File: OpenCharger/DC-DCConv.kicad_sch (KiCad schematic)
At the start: 10 parts, among them Q5 IPT015N10N5, Q6 IPT015N10N5, Q7 IPT015N10N5, Q9 IPT015N10N5, U4 IRS25606S

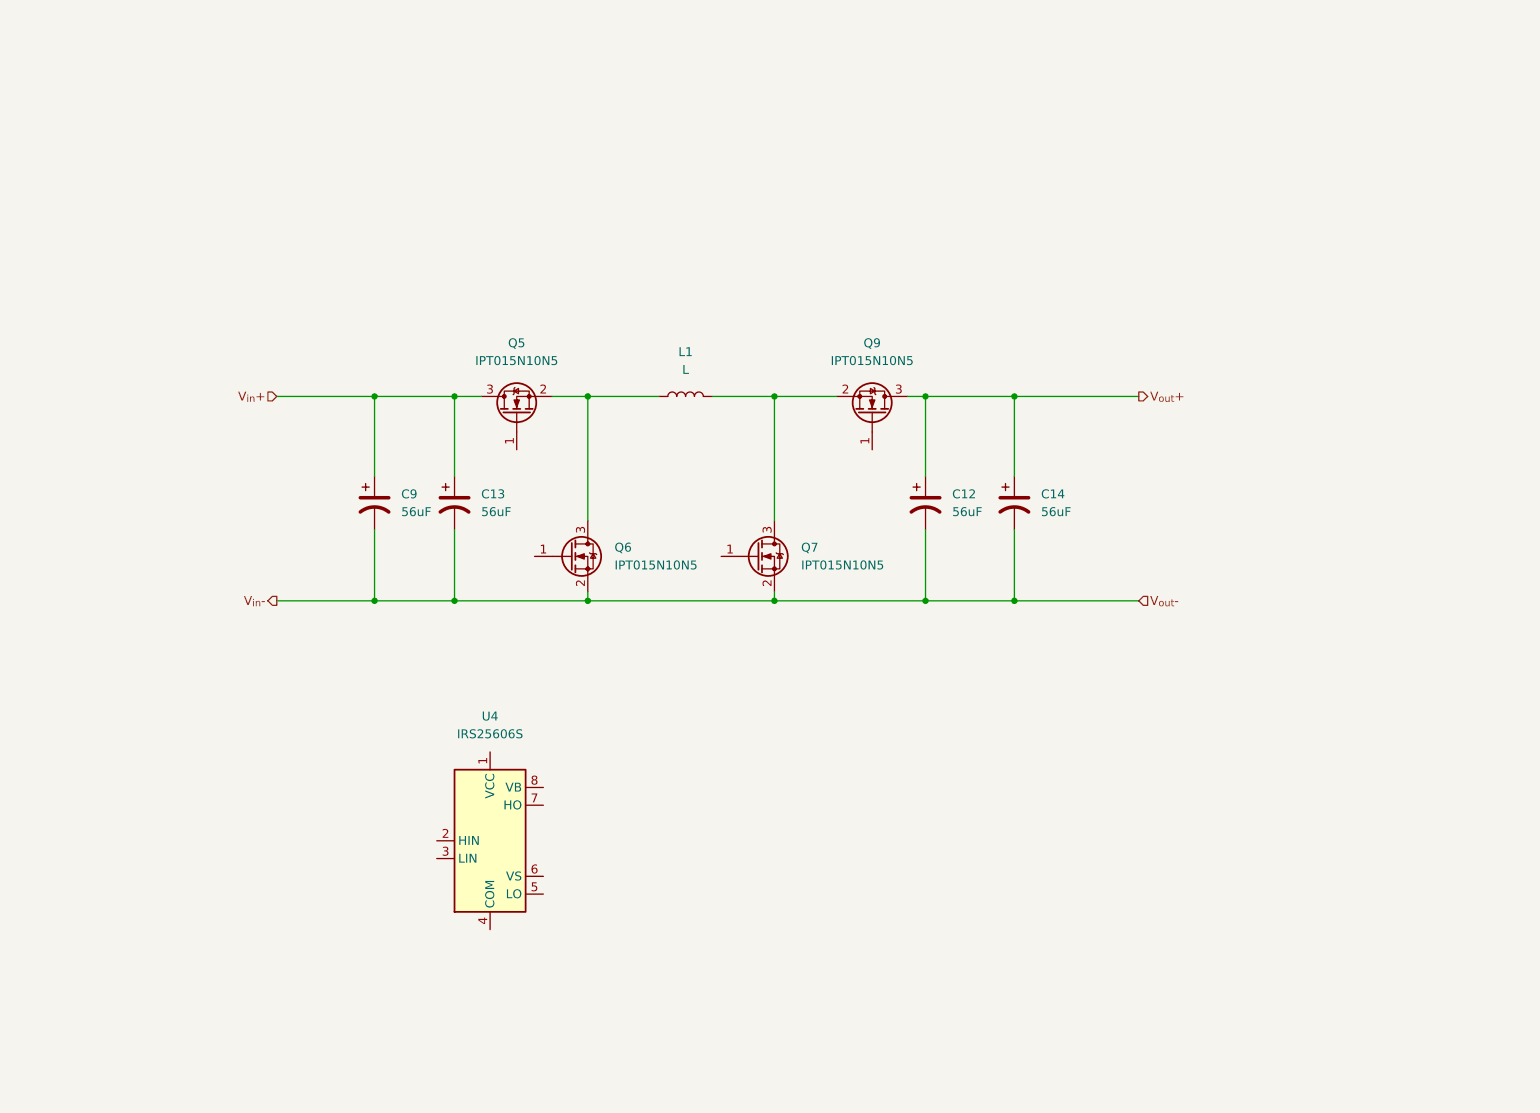
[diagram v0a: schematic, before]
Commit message: updated
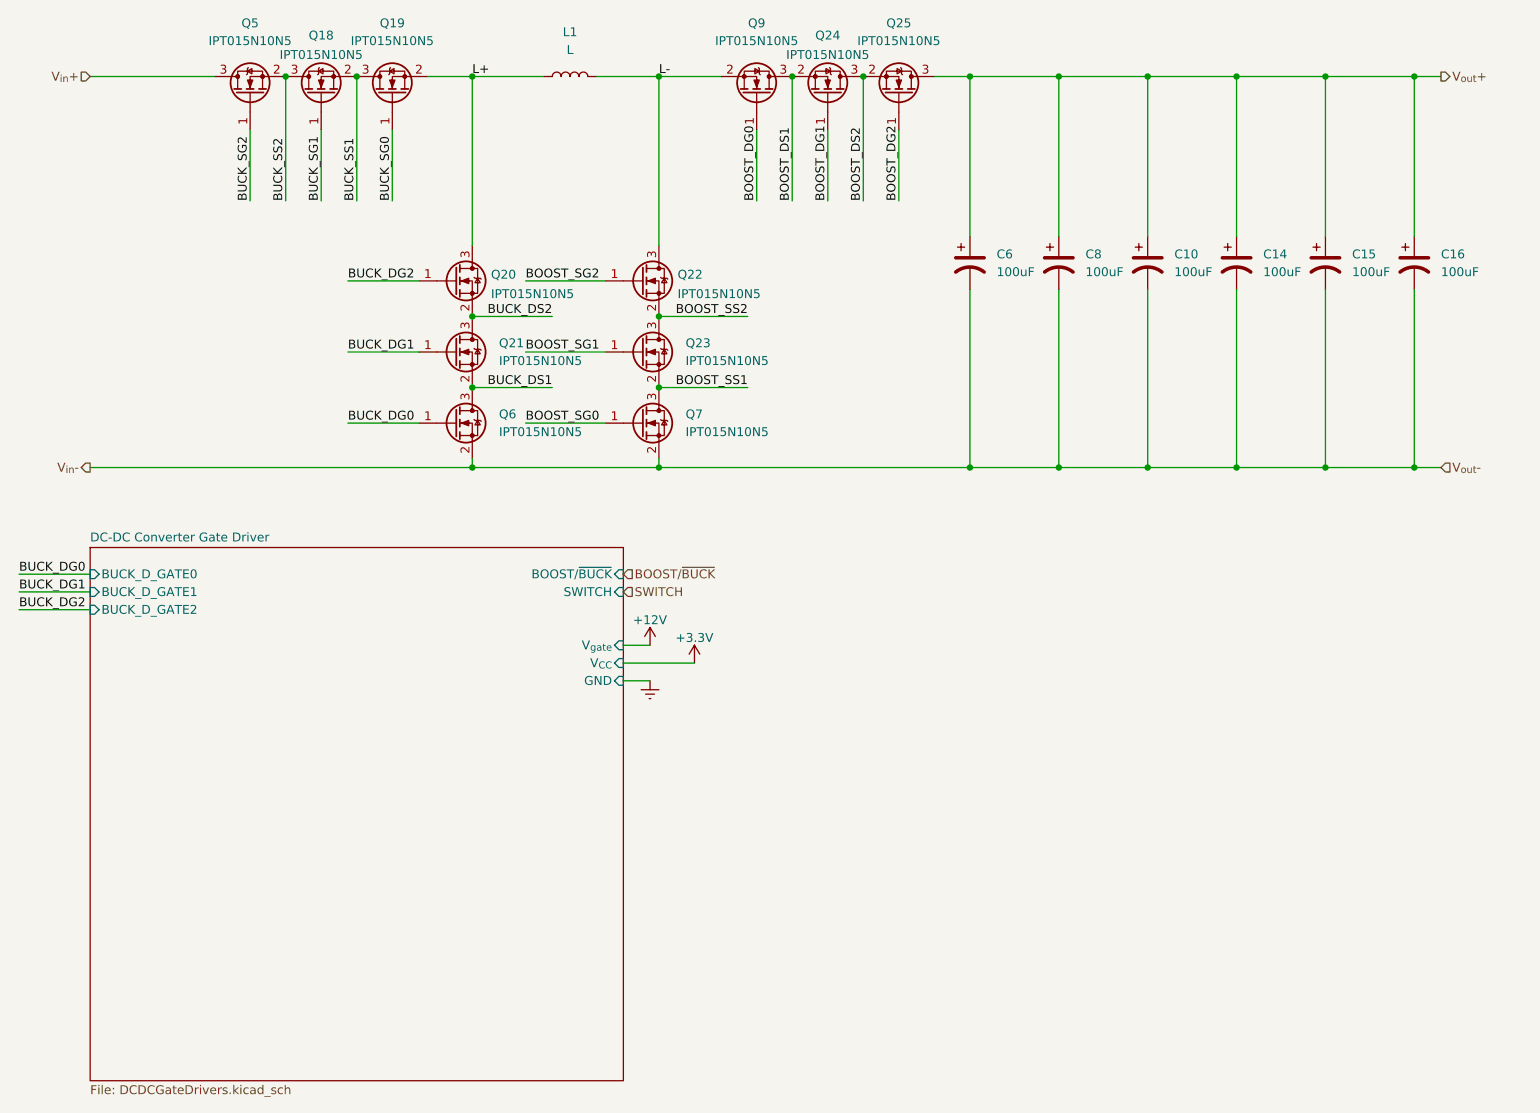
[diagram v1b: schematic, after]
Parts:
- removed C12, C13, C9: 56uF, Capacitor_THT:CP_Radial_D40.0mm_P10.00mm_SnapIn, symbol Device:C_Polarized_US
- removed U4: IRS25606S, Package_SO:SOIC-8_3.9x4.9mm_P1.27mm, symbol Driver_FET:IRS25606S
- added C10, C15, C16, C6, C8: 100uF, Capacitor_THT:CP_Radial_D16.0mm_P7.50mm, symbol Device:C_Polarized_US
- added Q18, Q19, Q20, Q21, Q22, Q23, Q24, Q25: IPT015N10N5, Package_TO_SOT_SMD:Infineon_PG-HSOF-8-1, symbol Transistor_FET:IPT015N10N5
- C14: value 56uF -> 100uF; footprint Capacitor_THT:CP_Radial_D40.0mm_P10.00mm_SnapIn -> Capacitor_THT:CP_Radial_D16.0mm_P7.50mm
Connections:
- net V_{in}-: now also C10.2, C15.2, C16.2, C6.2, C8.2
- net V_{out}+: now also C10.1, C15.1, C16.1, C6.1, C8.1, Q25.3 (D); no longer Q9.3 (D)
- net BOOST_SG0: now reaches Q7.1 (G)
- net L-: now reaches L1.2, Q9.2 (S)
- net L-: now also Q22.3 (D); no longer Q7.3 (D)
- net BUCK_DG0: now reaches Q6.1 (G)
- net BOOST_DG0: now reaches Q9.1 (G)
- net BUCK_SG2: now reaches Q5.1 (G)
- new net BOOST_DG1: Q24.1 (G)
- new net BOOST_DG2: Q25.1 (G)
- new net BOOST_DS1: Q24.2 (S), Q9.3 (D)
- new net BOOST_DS2: Q24.3 (D), Q25.2 (S)
- new net BOOST_SG1: Q23.1 (G)
- new net BOOST_SG2: Q22.1 (G)
- new net BOOST_SS1: Q23.2 (S), Q7.3 (D)
- new net BOOST_SS2: Q22.2 (S), Q23.3 (D)
- new net BUCK_DG1: Q21.1 (G)
- new net BUCK_DG2: Q20.1 (G)
- new net BUCK_DS1: Q21.2 (S), Q6.3 (D)
- new net BUCK_DS2: Q20.2 (S), Q21.3 (D)
- new net BUCK_SG0: Q19.1 (G)
- new net BUCK_SG1: Q18.1 (G)
- new net BUCK_SS1: Q18.2 (S), Q19.3 (D)
- new net BUCK_SS2: Q18.3 (D), Q5.2 (S)
- new net L+: L1.1, Q19.2 (S), Q20.3 (D)
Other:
- added sheet DC-DC Converter Gate Driver (DCDCGateDrivers.kicad_sch)
- moved on the sheet: L1, Q5, Q6, Q7, Q9
